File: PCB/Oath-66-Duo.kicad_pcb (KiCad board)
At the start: 2 copper layers, 349.1 x 99.1 mm, 154 parts, among them J1 GH1.25 Battery Connector, J2 GH1.25 Battery Connector, U1 nice_nano, U2 nice_nano

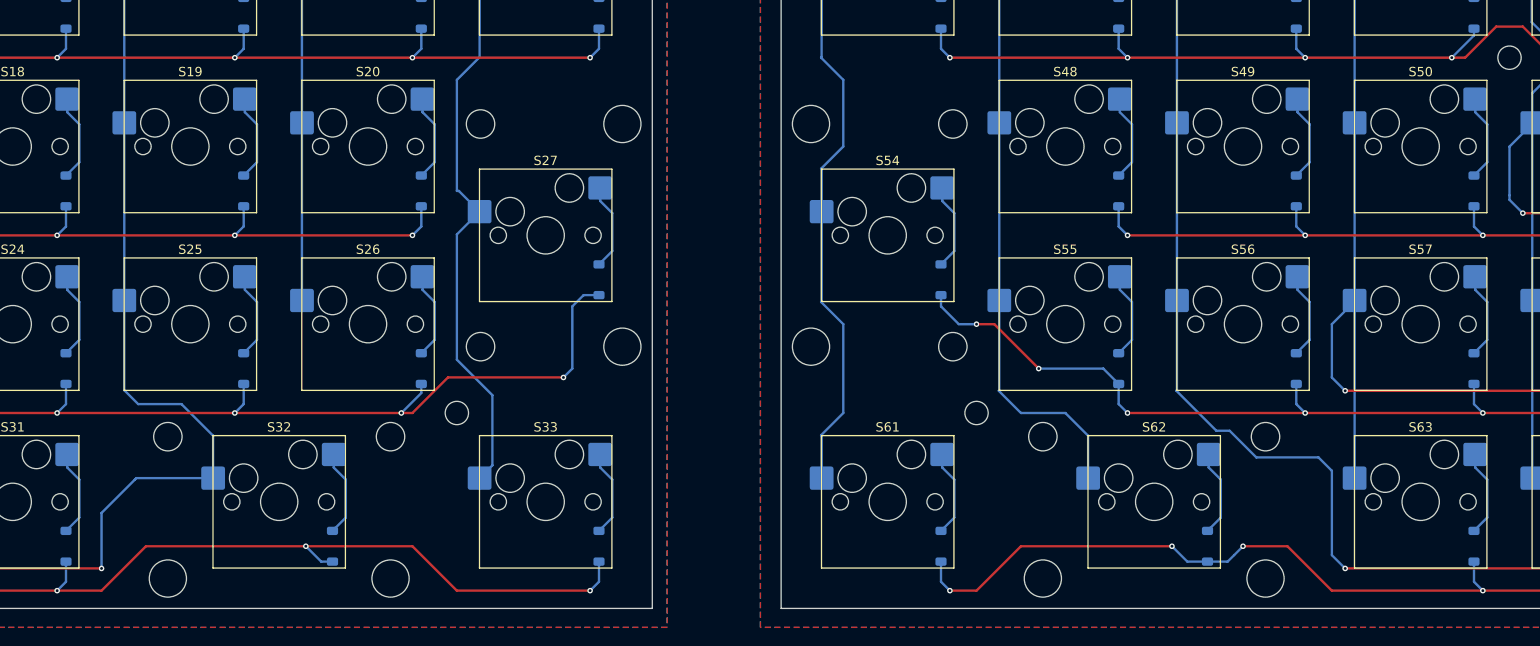
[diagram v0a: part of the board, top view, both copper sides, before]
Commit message: PCB Updated
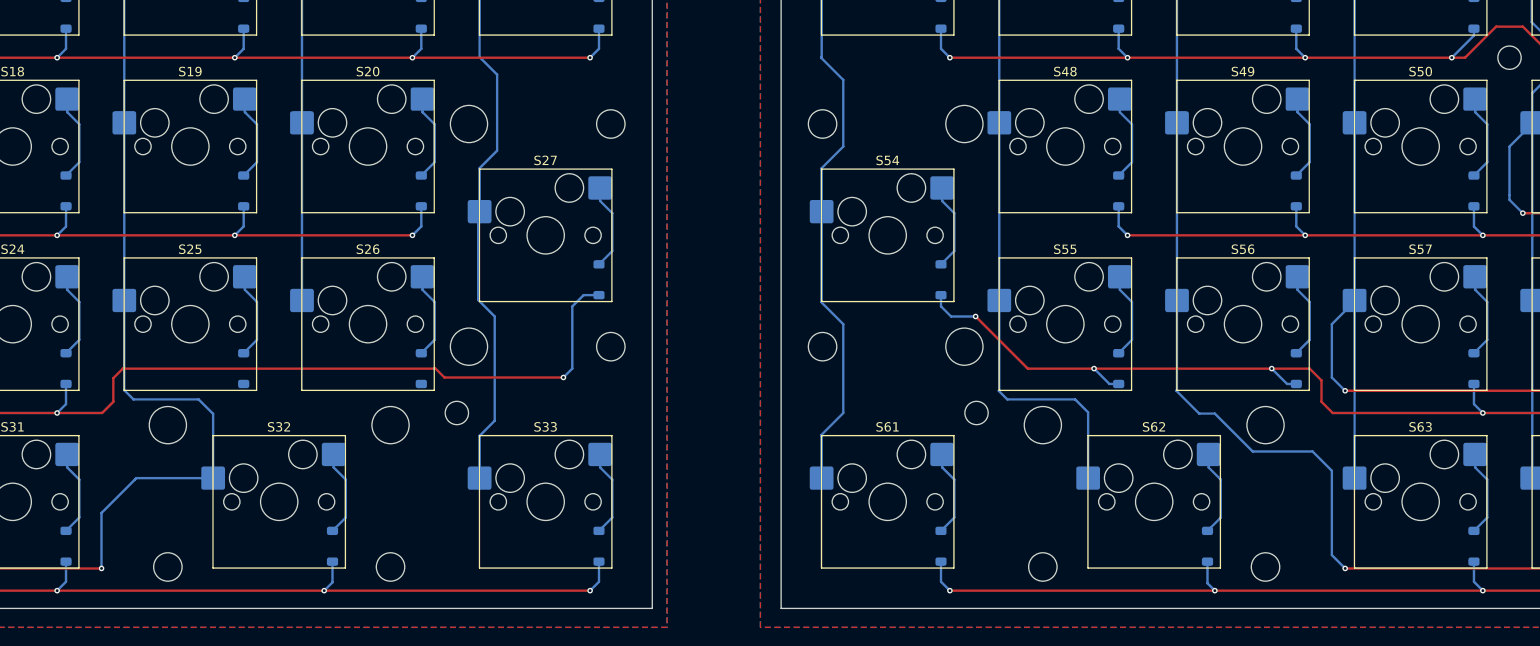
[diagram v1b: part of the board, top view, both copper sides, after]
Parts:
- turned REF** to -90 degrees
- turned REF** to 90 degrees
- turned REF** to 180 degrees (x2)
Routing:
- net ROW3_L: track 234.4 -> 229.2 mm, vias 9 -> 7
- net ROW4_L: track 235.9 -> 231.9 mm
- net ROW3_R: track 210.0 -> 213.2 mm, vias 10 -> 9
- net COL6_L: track 245.5 -> 243.3 mm
- net ROW4_R: track 222.7 -> 220.8 mm, vias 9 -> 8
- net COL1_R: track 238.3 -> 239.7 mm
- net COL4_L: track 260.1 -> 261.5 mm
